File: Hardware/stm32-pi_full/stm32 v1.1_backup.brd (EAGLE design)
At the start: 131.4 x 105.8 mm, 265 parts, among them IC1 TS461CLT, J1 JUMPER-SMT_2_NC_TRACE_NO-SILK, Q1 PNP, Q2 NPN, Q3 NPN, U1 ESP32-WROOM-32D, U2 RFM69HCW/RFM95W

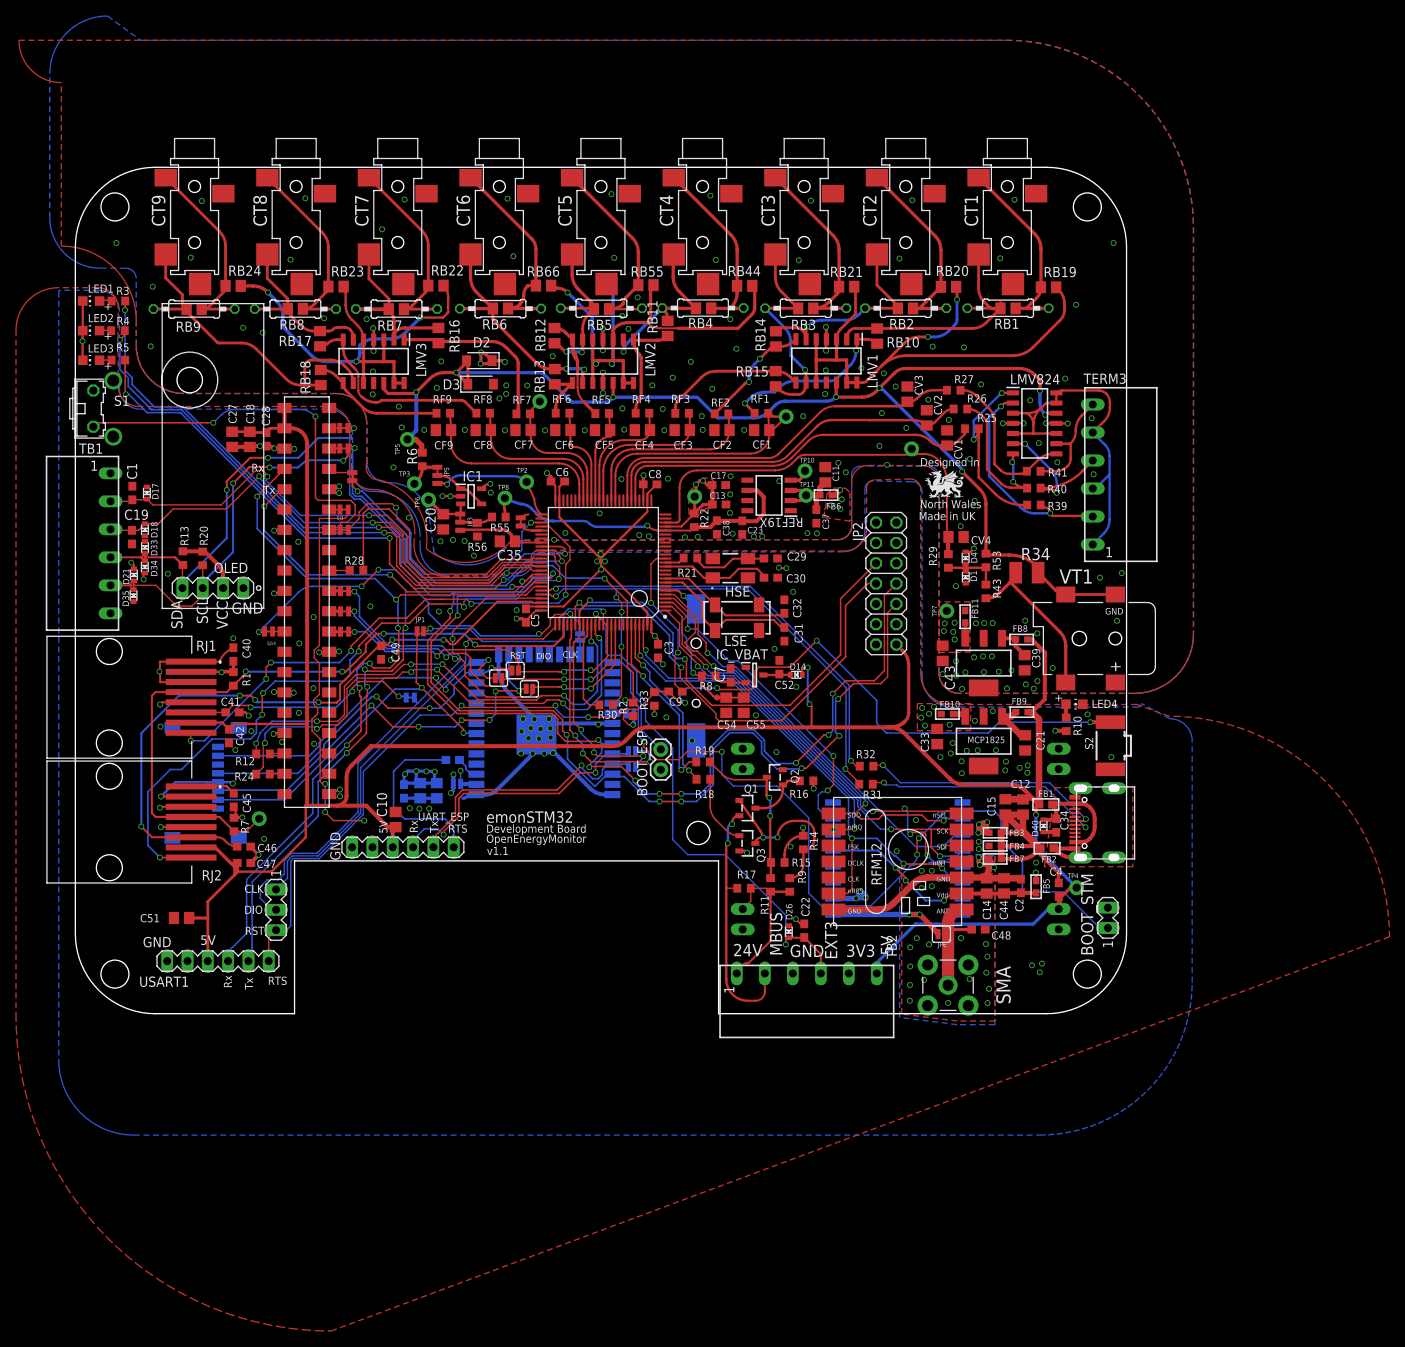
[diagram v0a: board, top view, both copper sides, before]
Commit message: tidy
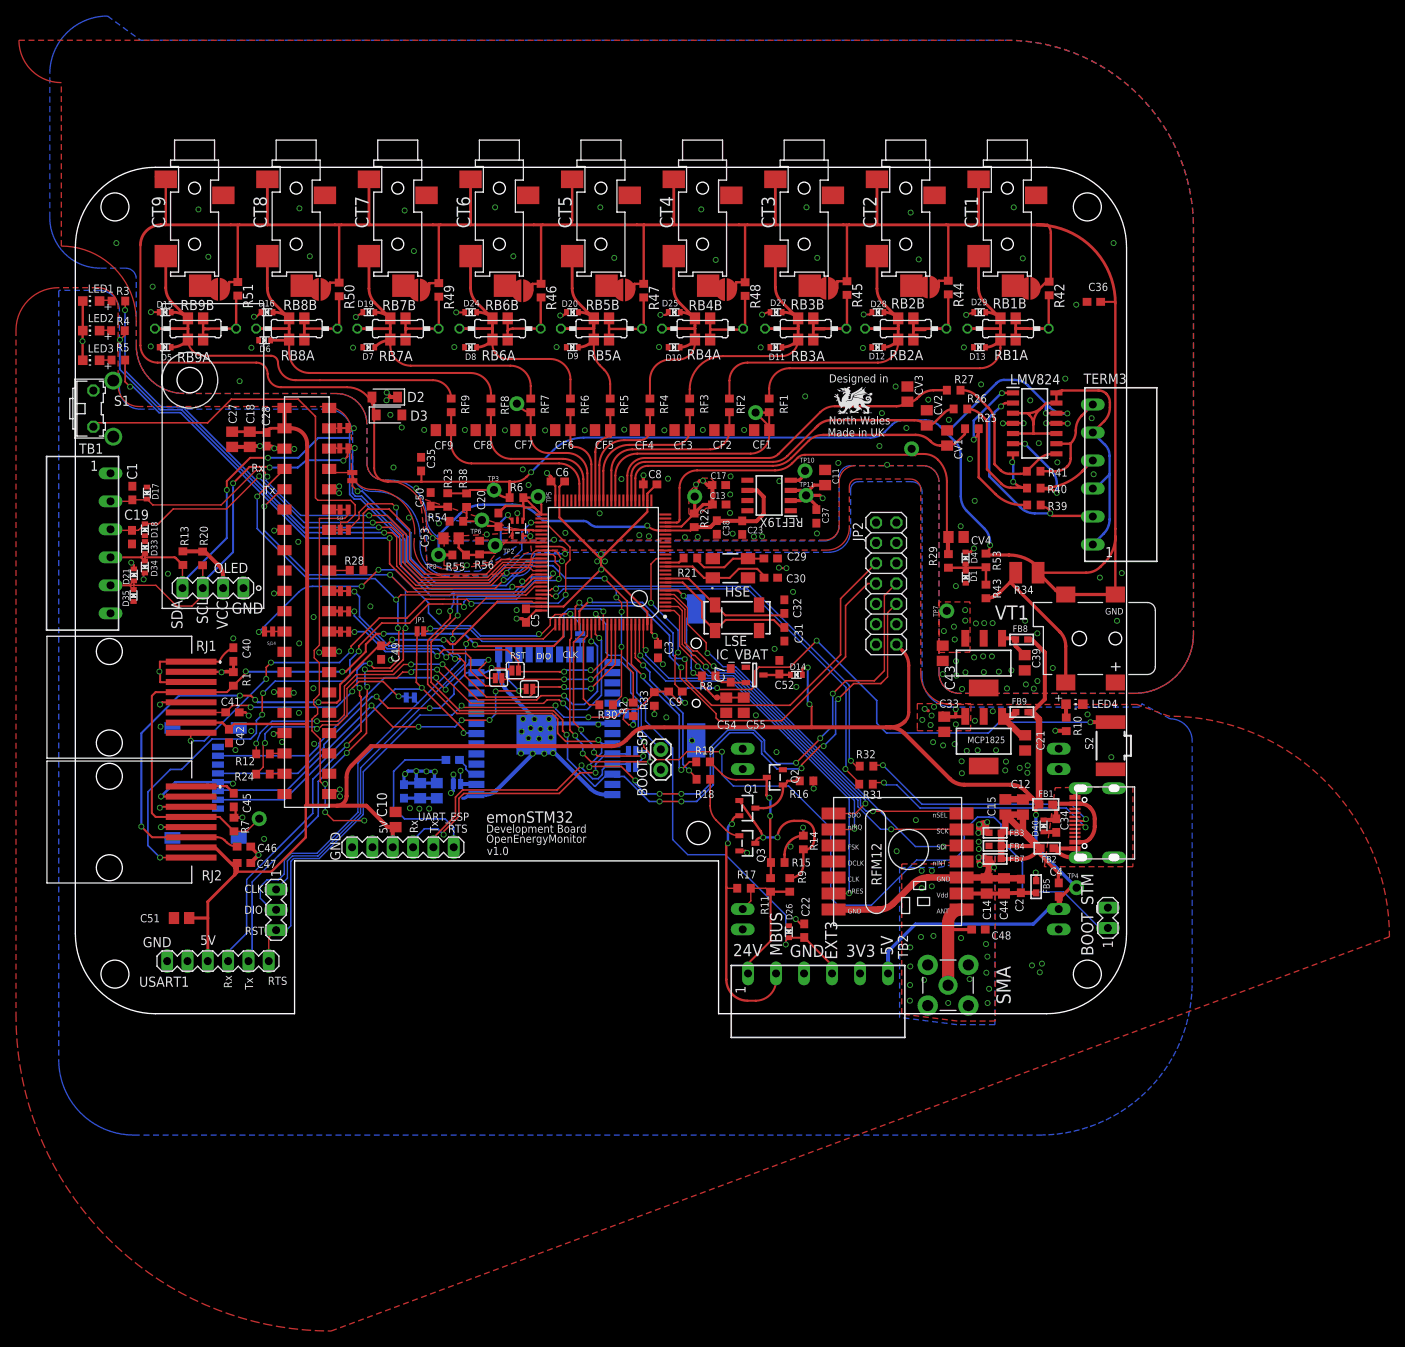
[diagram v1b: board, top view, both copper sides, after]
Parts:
- removed FB10, FB11, FB6: (no value), microbuilder:_0603
- removed IC1: TS461CLT, TS461CLT:SOT95P280X145-5N
- removed JP3, JP5: JUMPER-SMT_3_1-NC_TRACE_NO-SILK, SparkFun-Jumpers:SMT-JUMPER_3_1-NC_TRACE_NO-SILK
- removed JP6: JUMPER-SMT_2_NC_PASTE_SILK, SparkFun-Jumpers:SMT-JUMPER_2_NC_PASTE_SILK
- removed LMV1, LMV2, LMV3: LMV824IDG4, LMV824IDG4:SOIC127P600X175-14N
- removed RB1, RB2, RB3, RB4, RB5, RB6, RB7, RB8, RB9: 6R81, rcl:R0805
- removed RB10, RB11, RB12, RB13, RB14, RB15, RB16, RB17, RB18: 510R 0.1%, rcl:R0805
- removed RB19, RB20, RB21, RB22, RB23, RB24, RB44, RB55, RB66: 680R | 681R 0.1%, rcl:R0805
- removed SJ1: JUMPER-SMT_2_NC_TRACE_NO-SILK, SparkFun-Jumpers:SMT-JUMPER_2_NC_TRACE_NO-SILK
- removed U2: RFM69HCW/RFM95W, microbuilder:RFMHCW_SMT
- added C36: (no value), rcl:C0603
- added C50: 1uF, rcl:C0603
- added C53: 22uF, rcl:C0805
- added D10, D11, D12, D13, D15, D16, D19, D20, D24, D25, D27, D28, D29, D5, D6, D7, D8, D9: ESD5Z3.3T1G, microbuilder:SOD-523
- added IC2: (no value), analog-devices:SC70-5
- added JP10, JP11, JP12, JP13, JP14, JP15, JP16, JP17, JP18: JUMPER-SMT_2_NO_NO-SILK_ROUND, SparkFun-Jumpers:SMT-JUMPER_2_NO_NO-SILK_ROUND
- added R23: 1k, resistor:R0603
- added R38: 39k, resistor:R0603
- added R42, R44, R45, R46, R47, R48, R49, R50, R51: 0R, rcl:R0603
- added R54: 10k, resistor:R0603
- added RB1A, RB2A, RB3A, RB4A, RB5A, RB6A, RB7A, RB8A, RB9A: 6R8, rcl:R0805
- added RB1B, RB2B, RB3B, RB4B, RB5B, RB6B, RB7B, RB8B, RB9B: (no value), rcl:R0805
- C11, C23: value 22uf -> 1uF
- C20: value 22uF -> 2.2nF; device rcl:C0805 -> rcl:C0603
- C35: value 22uF -> (none); device rcl:C0805 -> rcl:C0603
- FB1: value 1600R -> (none)
- FB2: value 0R -> (none)
- R55: value 10k -> 91k
- R6: value 20R -> 0R; device rcl:R0603 -> resistor:R0603
- moved TP5 17.8 mm to (57.8, 64.6)
- moved C35 14.5 mm to (43.2, 68.7), turned to 90 degrees
- moved R6 12.7 mm to (55.1, 64.5), turned to 180 degrees
- moved D2 12.7 mm to (38.7, 77.1)
- moved D3 12.1 mm to (39.2, 74.8)
- moved TP8 10.9 mm to (45.4, 57.3)
- moved TP3 9.98 mm to (52.3, 65.5)
- moved TP2 8.85 mm to (52.5, 58.5)
- moved TP6 7.12 mm to (50.8, 61.7)
- moved C20 6.90 mm to (52.9, 61.7), turned to 90 degrees
- moved R55 6.86 mm to (48.0, 57.3), turned to 180 degrees
- moved TP18 3.84 mm to (85.0, 75.1)
- moved TP19 2.88 mm to (55.2, 76.3)
- moved RB4_ 2.57 mm to (78.4, 85.6)
- moved RB1_ 2.54 mm to (116.6, 85.6)
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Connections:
- net CT1_ADC renamed CT1
- net CT2_ADC renamed CT2
- net CT3_ADC renamed CT3
- net CT4_ADC renamed CT4
- net CT5_ADC renamed CT5
- net CT6_ADC renamed CT6
- removed net ANT_LORA: JP6.1, U2.1P
- removed net BIAS123: LMV1.10, LMV1.13, LMV1.14, LMV1.3, LMV1.5, RB19.2, RB20.2, RB21.2
- removed net BIAS456: LMV2.10, LMV2.13, LMV2.14, LMV2.3, LMV2.5, RB44.2, RB55.2, RB66.2
- removed net BIAS789: LMV3.10, LMV3.13, LMV3.14, LMV3.3, LMV3.5, RB22.2, RB23.2, RB24.2
- removed net BIAS_SOT23: IC1.1, IC1.4, JP5.2
- removed net CT1_OUT: LMV1.1, RB10.1, RF1.1
- removed net CT2_OUT: LMV1.7, RB14.1, RF2.1
- removed net CT3_OUT: LMV1.8, RB15.2, RF3.1
- removed net CT4_OUT: LMV2.1, RB11.1, RF4.1
- removed net CT5_OUT: LMV2.7, RB12.1, RF5.1
- removed net CT6_OUT: LMV2.8, RB13.2, RF6.1
- removed net CT7_OUT: LMV3.1, RB16.1, RF7.1
- removed net CT8_OUT: LMV3.7, RB17.1, RF8.1
- removed net CT9_OUT: LMV3.8, RB18.2, RF9.1
- removed net DIO1_RFM: STM32F303VE.3, U2.7P
- removed net N$12: CT5.P$3
- removed net N$38: CT4.P$3
- removed net N$39: C20.1, IC1.3, JP3.3, TP6.1
- removed net N$40: CT6.P$1, RB6.2, RB66.1, RB6_.2
- removed net N$42: JP5.3, R6.1, TP3.1
- removed net N$43: CT9.P$1, RB24.1, RB9.2, RB9_.2
- removed net N$45: CT8.P$1, RB23.1, RB8.2, RB8_.2
- removed net N$46: CT7.P$1, RB22.1, RB7.2, RB7_.2
- removed net STM32_OPAMP_NON-INVERT+: C35.1, JP3.1, STM32F303VE.58
- removed net STM32_OPAMP_OUT: JP5.1, STM32F303VE.51, TP2.1
- new net OPAMP_NON-INVERT+: C53.1, IC2.3, R55.1, R56.2, STM32F303VE.58, TP2.1
- net +3V3: now also MCP1825.3; no longer FB10.2
- net +3V3ANA: now also C11.1, C37.1, D15.K, D16.K, D19.K, D20.K, D24.K, D25.K, D27.K, D28.K, D29.K, IC2.5, MCP1825(ANALOG).3, REF19X.2, REF19X.3, TP11.1; no longer FB11.2, FB6.2, IC1.2, LMV1.4, LMV2.4, LMV3.4
- net AGND: now also C36.2, C50.2, C53.2, D10.A, D11.A, D12.A, D13.A, D5.A, D6.A, D7.A, D8.A, D9.A, IC2.2, R54.2; no longer C20.2, IC1.5, LMV1.11, LMV2.11, LMV3.11
- net ANT: no longer JP6.2
- net BIAS: now also C35.1, C36.1, CT1.P$1, CT2.P$1, CT3.P$1, CT4.P$1, CT5.P$1, CT6.P$1, CT7.P$1, CT8.P$1, CT9.P$1, JP10.1, JP11.1, JP12.1, JP13.1, JP14.1, JP15.1, JP16.1, JP17.1, JP18.1, R23.2, R38.1, R42.1, R44.1, R45.1, R46.1, R47.1, R48.1, R49.1, R50.1, R51.1, TP3.1; no longer LMV1.12, LMV2.12, LMV3.12, TP5.1
- net CT_IN1: now also D13.K, D29.A, RB1A.1, RB1B.1, RF1.1; no longer LMV1.2, RB1.1, RB10.2
- net CT_IN2: now also D12.K, D28.A, RB2A.1, RB2B.1, RF2.1; no longer LMV1.6, RB14.2, RB2.1
- net CT_IN3: now also D11.K, D27.A, RB3A.1, RB3B.1, RF3.1; no longer LMV1.9, RB15.1, RB3.1
- net CT_IN4: now also D10.K, D25.A, RB4A.1, RB4B.1, RF4.1; no longer LMV2.2, RB11.2, RB4.1
- net CT_IN5: now also D20.A, D9.K, RB5A.1, RB5B.1, RF5.1; no longer LMV2.6, RB12.2, RB5.1
- net CT_IN6: now also D24.A, D8.K, RB6A.1, RB6B.1, RF6.1; no longer LMV2.9, RB13.1, RB6.1
- net CT_IN7: now also D19.A, D7.K, RB7A.1, RB7B.1, RF7.1; no longer LMV3.2, RB16.2, RB7.1
- net CT_IN8: now also D16.A, D6.K, RB8A.1, RB8B.1, RF8.1; no longer LMV3.6, RB17.2, RB8.1
- net CT_IN9: now also D15.A, D5.K, RB9A.1, RB9B.1, RF9.1; no longer LMV3.9, RB18.1, RB9.1
- net DGND: no longer U2.9P
- net DIO0_RFM: no longer U2.6P
- net N$1: now also JP10.2
- net N$10: now also JP13.2
- net N$13: now also JP14.2
- net N$2: now also JP11.2
- net N$20: now also JP15.2
- net N$21: now also JP16.2
- net N$22: now also JP17.2
- net N$23: now also JP18.2
- net N$24: now also R47.2, RB5A.2, RB5B.2, RB5_.2; no longer CT6.P$3
- net N$25: now also R46.2, RB6A.2, RB6B.2, RB6_.2; no longer FB10.1, MCP1825.3
- net N$26: now also R42.2, RB1A.2, RB1B.2; no longer CT1.P$1, RB1.2, RB19.1
- net N$27: now also R44.2, RB2A.2, RB2B.2; no longer CT2.P$1, RB2.2, RB20.1
- net N$29: now also R50.2, RB8A.2, RB8B.2, RB8_.2; no longer C11.1, C37.1, FB6.1, REF19X.2, REF19X.3, TP11.1
- net N$34: now also R51.2, RB9A.2, RB9B.2, RB9_.2; no longer FB11.1, MCP1825(ANALOG).3
- net N$35: now also R48.2, RB4A.2, RB4B.2; no longer CT4.P$1, RB4.2, RB44.1
- net N$36: now also R49.2, RB7A.2, RB7B.2, RB7_.2; no longer CT3.P$1, RB21.1, RB3.2, RB3_.2
- net N$37: now also R45.2, RB3A.2, RB3B.2, RB3_.2; no longer JP3.2, R55.1, R56.2
- net N$7: now also C50.1, R23.1; no longer CT5.P$1, RB5.2, RB55.1, RB5_.2
- net N$8: now also JP12.2
- net OPAMP_INVERT-: now also C20.1, IC2.4, R38.2, R54.1, TP6.1; no longer SJ1.1
- net OPAMP_OUT: now also C20.2, IC2.1, R6.1, STM32F303VE.51, TP5.1; no longer SJ1.2
- net RGND: no longer U2.16P, U2.2P
- net RST_RFM: no longer U2.14P
- net SPI4_CLK_MASTER: no longer U2.12P
- net SPI4_CS_RFM69_MASTER: no longer U2.13P
- net SPI4_MISO_MASTER: no longer U2.10P
- net SPI4_MOSI_MASTER: no longer U2.11P
- net VDD: no longer U2.5P
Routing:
- net BIAS: track 159.3 -> 525.0 mm, vias 8 -> 4
- net BIAS123: track 71.8 -> 0.00 mm, vias 2 -> 0
- net BIAS456: track 68.0 -> 0.00 mm, vias 3 -> 0
- net BIAS789: track 61.6 -> 0.00 mm, vias 3 -> 0
- net DIO1_RFM: track 39.9 -> 0.00 mm, vias 3 -> 0
- net +3V3ANA: track 40.1 -> 73.2 mm, vias 25 -> 23
- net CT_IN8: track 22.5 -> 49.6 mm
- net N$40: track 26.0 -> 0.00 mm
- net CT8_OUT: track 26.0 -> 0.00 mm
- net N$45: track 25.2 -> 0.00 mm
- net N$43: track 25.0 -> 0.00 mm
- net N$46: track 24.9 -> 0.00 mm
- net N$7: track 25.9 -> 2.18 mm
- net CT1_OUT: track 22.5 -> 0.00 mm, vias 2 -> 0
- net CT7_OUT: track 22.4 -> 0.00 mm
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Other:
- board text added: "v1.0"
- board text removed: "v1.1"
